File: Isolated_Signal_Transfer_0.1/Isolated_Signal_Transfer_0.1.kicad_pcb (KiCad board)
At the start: 2 copper layers, 54 x 20 mm, 22 parts, among them J1 Conn_01x02_Male, J2 Conn_01x02_Male, J3 Conn_01x04, U1 LM358, U2 IL300, U3 LM358

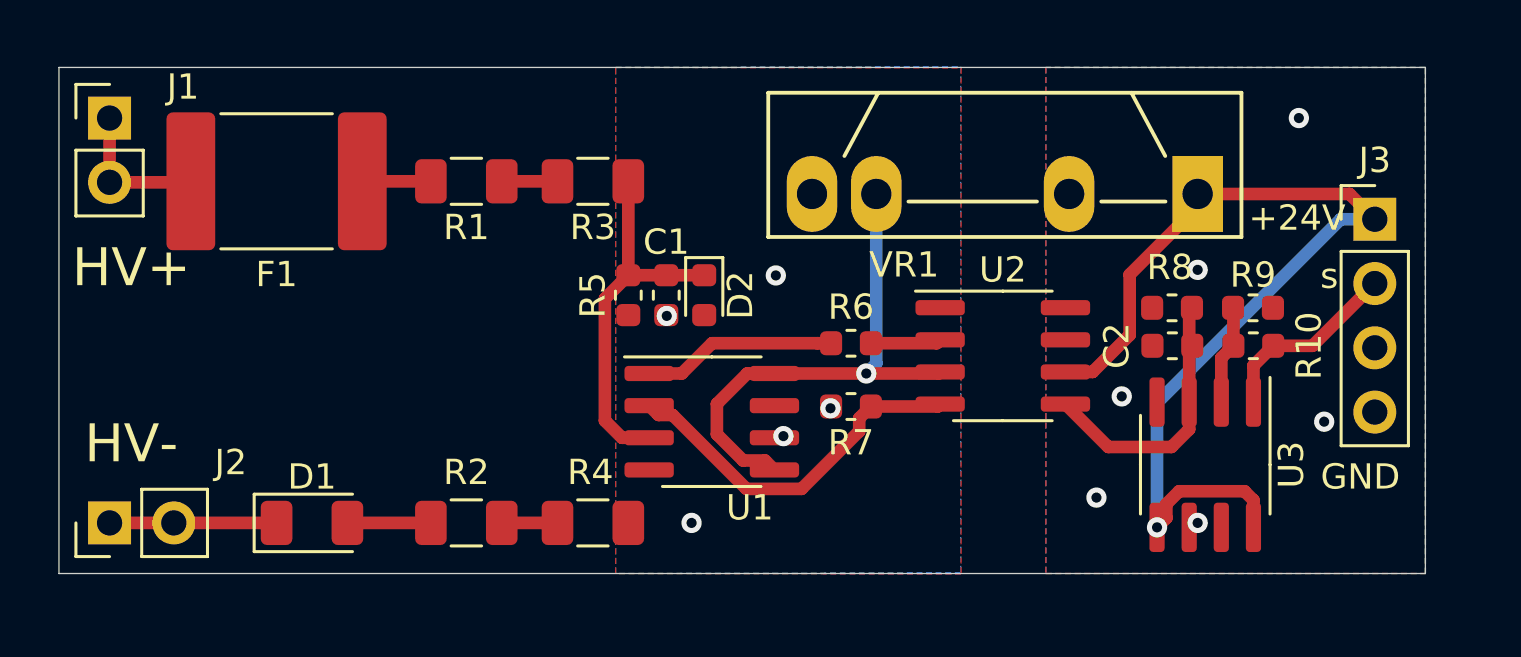
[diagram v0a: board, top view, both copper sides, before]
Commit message: Changes
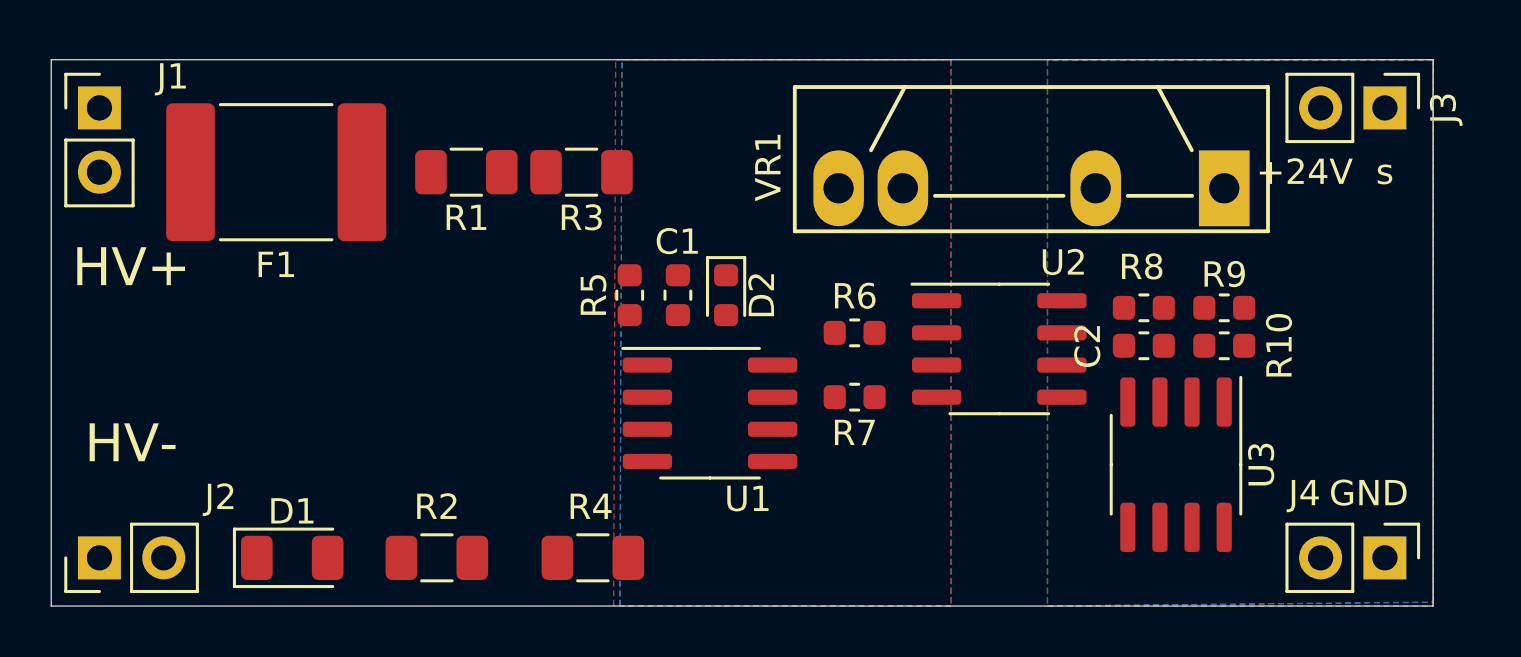
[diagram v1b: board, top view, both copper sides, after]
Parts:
- added J4: Conn_01x02_Male, Connector_PinHeader_2.54mm:PinHeader_1x02_P2.54mm_Vertical, F.Cu at (152.4, 119.4)
- J3: value Conn_01x04 -> Conn_01x02_Male; footprint Connector_PinHeader_2.54mm:PinHeader_1x04_P2.54mm_Vertical -> Connector_PinHeader_2.54mm:PinHeader_1x02_P2.54mm_Vertical
- moved J3 4.42 mm to (152.4, 101.6), turned to 270 degrees
- moved R2 1.81 mm to (114.9, 119.4)
- moved D1 1.59 mm to (109.2, 119.4)
- moved J2 1.44 mm to (101.6, 119.4)
- moved R4 1.38 mm to (121.1, 119.4)
- moved U3 1.16 mm to (144.1, 115.7)
- moved R10 1.15 mm to (146.1, 111.0)
- moved R9 1.14 mm to (146.1, 109.5)
- moved C2 1.12 mm to (142.9, 111.0)
- moved R8 1.11 mm to (142.9, 109.5)
- moved VR1 1.07 mm to (146.1, 104.8)
- moved D2 0.86 mm to (126.4, 109.0)
- moved R3 0.58 mm to (120.7, 104.1)
- moved J1 0.57 mm to (101.6, 101.6)
- moved C1 0.46 mm to (124.5, 109.0)
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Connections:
- J3 pad 1: +24V -> Net-(J3-Pad1)
- J3 pad 2: Net-(J3-Pad2) -> +24V
- R10 pad 1: Net-(J3-Pad2) -> Net-(J3-Pad1)
- U3 pad 1: Net-(J3-Pad2) -> Net-(J3-Pad1)
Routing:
- net +24V: track 39.7 -> 0.00 mm, vias 1 -> 0
- net +5Viso: track 20.7 -> 0.00 mm, vias 1 -> 0
- net Net-(C1-Pad1): track 14.9 -> 0.00 mm
- net Net-(R7-Pad1): track 14.6 -> 0.00 mm
- net Net-(C2-Pad1): track 10.7 -> 0.00 mm
- net Net-(R6-Pad1): track 7.68 -> 0.00 mm
- net Net-(J3-Pad2): track 7.58 -> 0.00 mm
- net Net-(D1-Pad1): track 6.60 -> 0.00 mm
- net Net-(F1-Pad2): track 5.77 -> 0.00 mm
- net Net-(R10-Pad2): track 3.93 -> 0.00 mm
- net Net-(D1-Pad2): track 3.30 -> 0.00 mm
- net Net-(R6-Pad2): track 2.79 -> 0.00 mm
- net Net-(F1-Pad1): track 2.71 -> 0.00 mm
- net Net-(R2-Pad1): track 2.20 -> 0.00 mm
- net Net-(R1-Pad1): track 2.20 -> 0.00 mm
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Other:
- board size 54 x 20 mm -> 54.6 x 21.6 mm
